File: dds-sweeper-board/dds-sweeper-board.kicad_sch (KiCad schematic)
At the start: 10 parts, among them J1 REF CLK, J2 3V3, J3 1V8, J4 Headers for AD9959 Eval Board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, J5 Trigger In, SW1 Pico Power Switch, U1 Pico, U3 5V->1V8 Linear Regulator

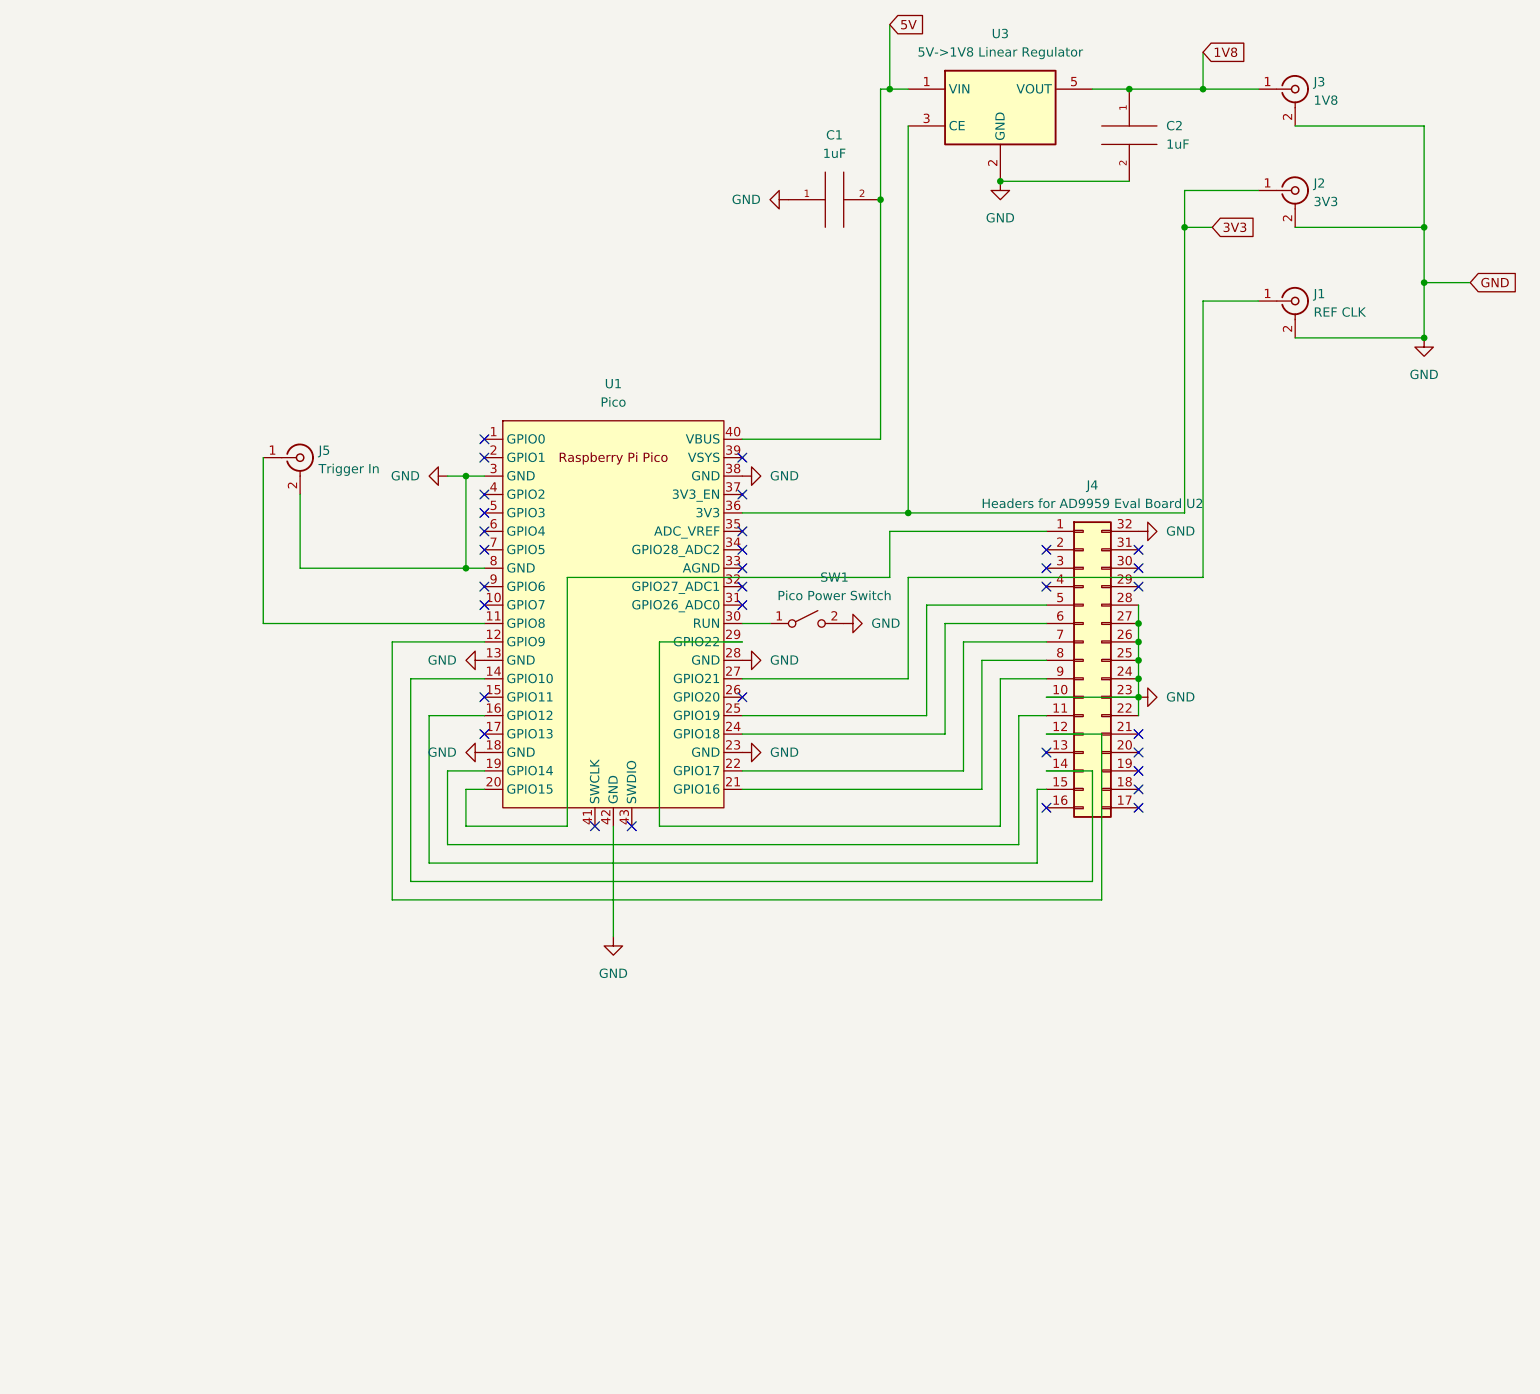
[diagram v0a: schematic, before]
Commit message: Updated board design
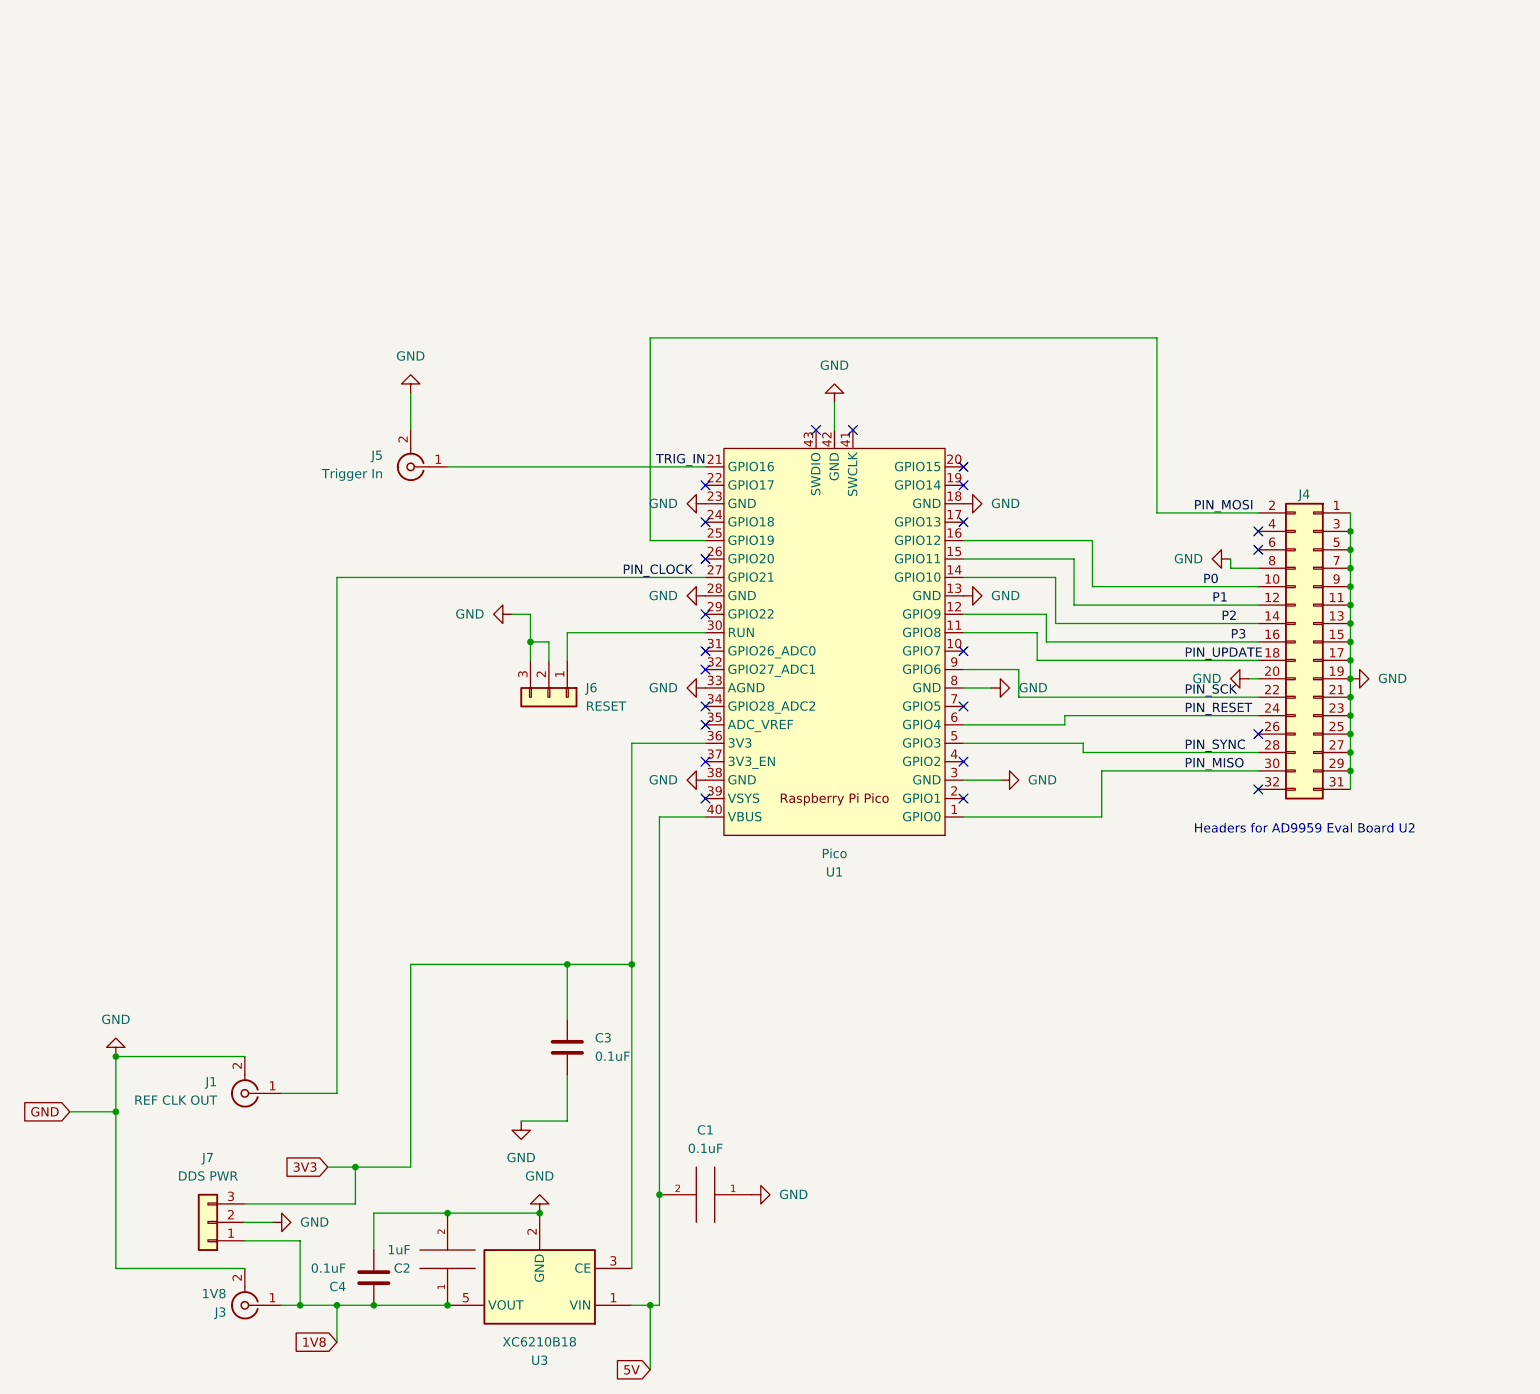
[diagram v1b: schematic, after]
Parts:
- removed J2: 3V3, Connector_Coaxial:SMA_Samtec_SMA-J-P-X-ST-EM1_EdgeMount, symbol Connector:Conn_Coaxial
- removed SW1: Pico Power Switch, Connector_PinSocket_2.54mm:PinSocket_1x03_P2.54mm_Vertical, symbol Switch:SW_SPST
- added C3, C4: 0.1uF, Capacitor_SMD:C_0805_2012Metric_Pad1.18x1.45mm_HandSolder, symbol Device:C
- added J6: RESET, Connector_PinSocket_2.54mm:PinSocket_1x03_P2.54mm_Vertical, symbol Connector_Generic:Conn_01x03
- added J7: DDS PWR, Connector_PinSocket_2.54mm:PinSocket_1x03_P2.54mm_Vertical, symbol Connector_Generic:Conn_01x03
- C1: value 1uF -> 0.1uF
- J1: value REF CLK -> REF CLK OUT
- J4: value Headers for AD9959 Eval Board U2 -> AD9959 Eval Header; footprint Custom_Conn:PinSocket_2x16_P2.54mm_Vertical_DDS_Sweeper -> Connector_PinSocket_2.54mm:PinSocket_2x16_P2.54mm_Vertical; symbol Connector_Generic:Conn_02x16_Counter_Clockwise -> Connector_Generic:Conn_02x16_Odd_Even
- U3: value 5V->1V8 Linear Regulator -> XC6210B18
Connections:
- net 1V8: now also C4.1, J7.1 (Pin_1)
- net 3V3: now also C3.2, J7.3 (Pin_3)
- net GND: now also J4.1 (Pin_1), J4.11 (Pin_11), J4.13 (Pin_13), J4.15 (Pin_15), J4.17 (Pin_17), J4.19 (Pin_19), J4.20 (Pin_20), J4.21 (Pin_21), J4.29 (Pin_29), J4.3 (Pin_3), J4.31 (Pin_31), J4.5 (Pin_5), J4.7 (Pin_7), J4.8 (Pin_8), J4.9 (Pin_9), U1.33 (AGND), C3.1, C4.2, J6.2 (Pin_2), J6.3 (Pin_3), J7.2 (Pin_2); no longer J4.10 (Pin_10), J4.22 (Pin_22), J4.24 (Pin_24), J4.26 (Pin_26), J4.28 (Pin_28), J4.32 (Pin_32)
- net PIN_MISO: now reaches U1.1 (GPIO0)
- net PIN_MISO: now also J4.30 (Pin_30)
- net PIN_UPDATE: now reaches U1.11 (GPIO8)
- net PIN_UPDATE: now also J4.18 (Pin_18); no longer J5.1 (In)
- net P1: now reaches J4.12 (Pin_12)
- net P1: now also U1.15 (GPIO11); no longer U1.12 (GPIO9)
- net P2: now reaches J4.14 (Pin_14), U1.14 (GPIO10)
- net P0: now reaches U1.16 (GPIO12)
- net P0: now also J4.10 (Pin_10); no longer J4.15 (Pin_15)
- net at U1.19 (GPIO14): no longer J4.11 (Pin_11)
- net at U1.20 (GPIO15): no longer J4.1 (Pin_1)
- net TRIG_IN: now reaches U1.21 (GPIO16)
- net TRIG_IN: now also J5.1 (In); no longer J4.8 (Pin_8)
- net at U1.22 (GPIO17): no longer J4.7 (Pin_7)
- net at U1.24 (GPIO18): no longer J4.6 (Pin_6)
- net PIN_MOSI: now reaches U1.25 (GPIO19)
- net PIN_MOSI: now also J4.2 (Pin_2); no longer J4.5 (Pin_5)
- net PIN_CLOCK: now reaches J1.1 (In), U1.27 (GPIO21)
- net at U1.29 (GPIO22): no longer J4.9 (Pin_9)
- net at U1.30 (RUN): now also J6.1 (Pin_1)
- net PIN_SYNC: now reaches U1.5 (GPIO3)
- net PIN_SYNC: now also J4.28 (Pin_28)
- net PIN_RESET: now reaches U1.6 (GPIO4)
- net PIN_RESET: now also J4.24 (Pin_24)
- net PIN_SCK: now reaches U1.9 (GPIO6)
- net PIN_SCK: now also J4.22 (Pin_22)
- net P3: now reaches J4.16 (Pin_16)
- net P3: now also U1.12 (GPIO9)
- no-connect marks 33 -> 23
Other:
- note added: "Headers for AD9959 Eval Board U2"
- moved on the sheet: C1, C2, J1, J3, J4, J5, U1, U3
